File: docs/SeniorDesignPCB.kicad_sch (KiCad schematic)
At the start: 22 parts, among them J1 Conn_02x05_Odd_Even, SW1 RotaryEncoder_Switch, SW2 RotaryEncoder_Switch, SW3 SW_Push, U2 STM32F446RETx, U3 RC1602A, U4 MAX7375AXR805

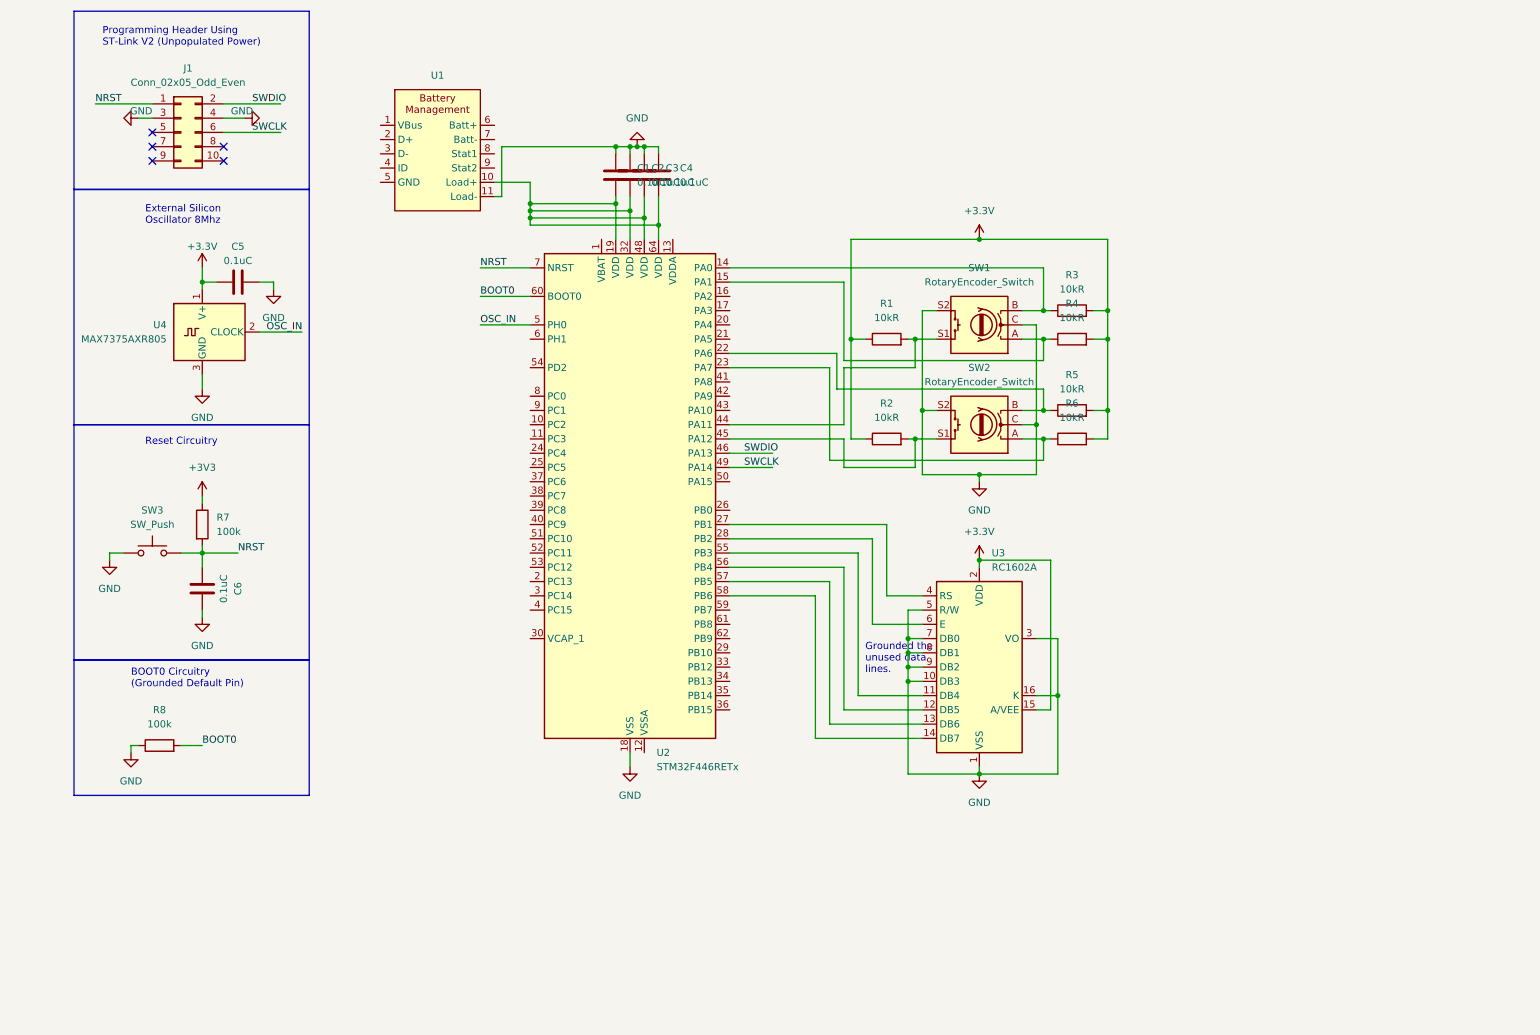
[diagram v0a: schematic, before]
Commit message: Add files via upload
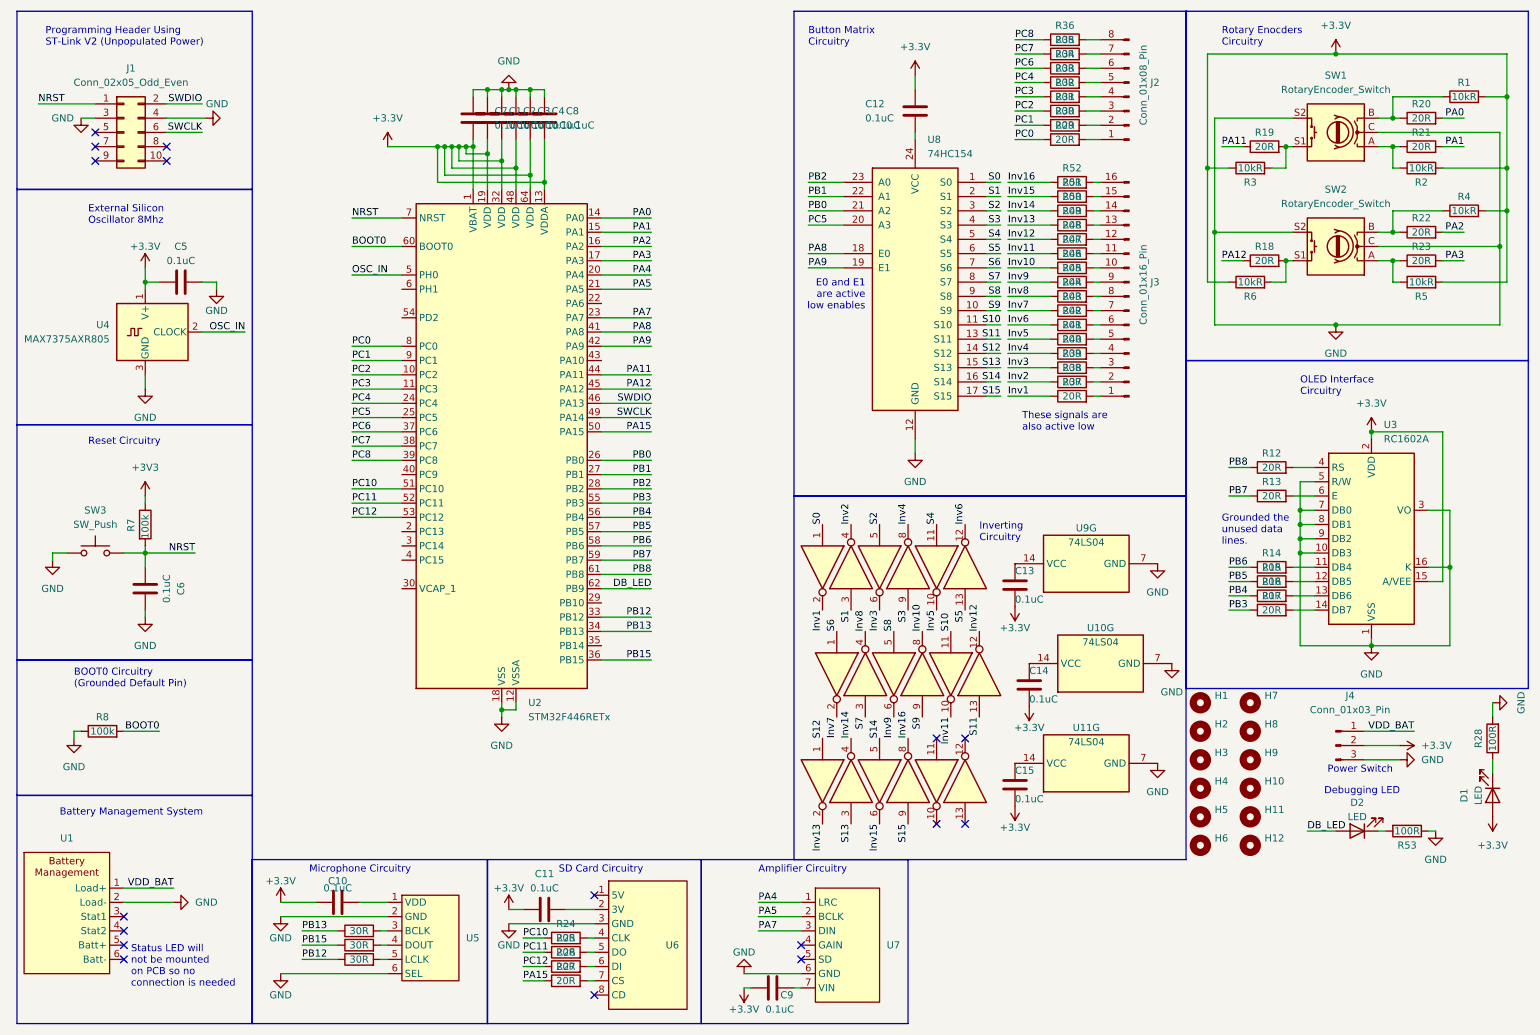
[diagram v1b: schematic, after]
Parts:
- added C10, C11, C12, C13, C14, C15, C7, C8, C9: 0.1uC, Capacitor_SMD:C_0805_2012Metric_Pad1.18x1.45mm_HandSolder, symbol Device:C
- added D1: LED, Diode_THT:D_5KP_P7.62mm_Vertical_AnodeUp, symbol Device:LED
- added D2: LED, Diode_SMD:D_0805_2012Metric, symbol Device:LED
- added H1, H2, H3, H4, H5, H6, H7, H8: MountingHole, MountingHole:MountingHole_2.2mm_M2, symbol Mechanical:MountingHole
- added H10, H11, H12, H9: MountingHole, MountingHole:MountingHole_2.5mm, symbol Mechanical:MountingHole
- added J2: Conn_01x08_Pin, Connector_PinHeader_2.54mm:PinHeader_1x08_P2.54mm_Vertical, symbol Connector:Conn_01x08_Pin
- added J3: Conn_01x16_Pin, Connector_PinHeader_2.54mm:PinHeader_1x16_P2.54mm_Vertical, symbol Connector:Conn_01x16_Pin
- added J4: Conn_01x03_Pin, Connector_PinHeader_2.54mm:PinHeader_1x03_P2.54mm_Vertical, symbol Connector:Conn_01x03_Pin
- added R10, R11, R9: 30R, Resistor_SMD:R_0805_2012Metric_Pad1.20x1.40mm_HandSolder, symbol Device:R
- added R12, R13, R14, R15, R16, R17, R18, R19, R20, R21, R22, R23, R24, R25, R26, R27, R29, R30, R31, R32, R33, R34, R35, R36, R37, R38, R39, R40, R41, R42, R43, R44, R45, R46, R47, R48, R49, R50, R51, R52: 20R, Resistor_SMD:R_0805_2012Metric_Pad1.20x1.40mm_HandSolder, symbol Device:R
- added R28, R53: 100R, Resistor_SMD:R_0805_2012Metric_Pad1.20x1.40mm_HandSolder, symbol Device:R
- added U10, U11, U9: 74LS04, Package_DIP:DIP-14_W7.62mm, symbol 74xx:74LS04
- added U5: ~, Connector_PinHeader_2.54mm:PinHeader_1x06_P2.54mm_Vertical, symbol SeniorDesignLibrary:MicrophoneBreakout
- added U6: ~, Connector_PinHeader_2.54mm:PinHeader_1x08_P2.54mm_Vertical, symbol SeniorDesignLibrary:SDBreakout
- added U7: ~, Connector_PinHeader_2.54mm:PinHeader_1x07_P2.54mm_Vertical, symbol SeniorDesignLibrary:Amplifier
- added U8: 74HC154, Package_DIP:DIP-24_W7.62mm, symbol 74xx:74LS154
- C1, C2, C3, C4, C5, C6: footprint Capacitor_SMD:C_1206_3216Metric_Pad1.33x1.80mm_HandSolder -> Capacitor_SMD:C_0805_2012Metric_Pad1.18x1.45mm_HandSolder
- J1: footprint Connector_PinHeader_1.00mm:PinHeader_2x05_P1.00mm_Vertical -> Connector_PinHeader_2.54mm:PinHeader_2x05_P2.54mm_Vertical
- SW3: footprint (none) -> Button_Switch_SMD:SW_Push_1P1T_NO_6x6mm_H9.5mm
- U1: footprint SeniorDesignFPLibrary:PCB_BatteryManagement -> Connector_PinHeader_2.54mm:PinHeader_1x06_P2.54mm_Vertical
- U3: footprint Display:RC1602A -> Connector_PinHeader_2.54mm:PinHeader_1x16_P2.54mm_Vertical
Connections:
- net +3.3V: now also C1.2, C2.2, C3.2, C4.2, R1.2, R2.2, R3.1, R6.1, U2.1 (VBAT), U2.13 (VDDA), U2.19 (VDD), U2.32 (VDD), U2.48 (VDD), U2.64 (VDD), C10.1, C11.1, C12.1, C13.2, C14.2, C15.2, C7.2, C8.2, C9.1, D1.2 (A), J4.2 (Pin_2); no longer R1.1, R2.1, R3.2, R6.2
- net GND: now also U1.2 (Load-), U2.12 (VSSA), C7.1, C8.1, J4.3 (Pin_3), R28.2, R53.1, U10.7 (GND), U11.7 (GND), U5.2 (GND), U5.6 (SEL), U6.3 (GND), U7.6 (GND), U8.12 (GND), U9.7 (GND); no longer U1.11 (Load-)
- net PC2: now reaches U2.10 (PC2)
- net PC2: now also R31.1
- net PC3: now reaches U2.11 (PC3)
- net PC3: now also R32.1
- net PA2: now reaches U2.16 (PA2)
- net PA2: now also R22.2
- net PA3: now reaches U2.17 (PA3)
- net PA3: now also R23.2
- net PA4: now reaches U2.20 (PA4)
- net PA4: now also U7.1 (LRC)
- net PA5: now reaches U2.21 (PA5)
- net PA5: now also U7.2 (BCLK)
- net PC4: now reaches U2.24 (PC4)
- net PC4: now also R33.1
- net PC5: now reaches U2.25 (PC5)
- net PC5: now also U8.20 (A3)
- net PB0: now reaches U2.26 (PB0)
- net PB0: now also U8.21 (A2)
- net at U3.4 (RS): now also R12.2; no longer U2.27 (PB1)
- net at U3.6 (E): now also R13.2; no longer U2.28 (PB2)
- net PB12: now reaches U2.33 (PB12)
- net PB12: now also R11.1
- net PB13: now reaches U2.34 (PB13)
- net PB13: now also R9.1
- net PB15: now reaches U2.36 (PB15)
- net PB15: now also R10.1
- net PC6: now reaches U2.37 (PC6)
- net PC6: now also R34.1
- net PC7: now reaches U2.38 (PC7)
- net PC7: now also R35.1
- net PC8: now reaches U2.39 (PC8)
- net PC8: now also R36.1
- net PA8: now reaches U2.41 (PA8)
- net PA8: now also U8.18 (E0)
- net PA9: now reaches U2.42 (PA9)
- net PA9: now also U8.19 (E1)
- net PA15: now reaches U2.50 (PA15)
- net PA15: now also R27.1
- net PC10: now reaches U2.51 (PC10)
- net PC10: now also R24.1
- net PC11: now reaches U2.52 (PC11)
- net PC11: now also R25.1
- net PC12: now reaches U2.53 (PC12)
- net PC12: now also R26.1
- net at U3.11 (DB4): now also R14.2; no longer U2.55 (PB3)
- net at U3.12 (DB5): now also R15.2; no longer U2.56 (PB4)
- net at U3.13 (DB6): now also R16.2; no longer U2.57 (PB5)
- net at U3.14 (DB7): now also R17.2; no longer U2.58 (PB6)
- net PB7: now reaches U2.59 (PB7)
- net PB7: now also R13.1
- net PB8: now reaches U2.61 (PB8)
- net PB8: now also R12.1
- net DB_LED: now reaches U2.62 (PB9)
- net DB_LED: now also D2.2 (A)
- net PC0: now reaches U2.8 (PC0)
- net PC0: now also R29.1
- net PC1: now reaches U2.9 (PC1)
- net PC1: now also R30.1
- net VDD_BAT: now reaches U1.1 (Load+)
- net VDD_BAT: now also J4.1 (Pin_1)
- new net: R19.2, R3.2, SW1.S1
- new net: J3.5 (Pin_5), R41.2
- new net: R22.1, R4.1, SW2.B
- new net: R24.2, U6.4 (CLK)
- new net: R27.2, U6.7 (CS)
- new net: J2.4 (Pin_4), R32.2
- new net: J3.1 (Pin_1), R37.2
- new net: J3.10 (Pin_10), R46.2
- new net: J3.11 (Pin_11), R47.2
- new net: J3.12 (Pin_12), R48.2
- new net: J3.13 (Pin_13), R49.2
- new net: J3.14 (Pin_14), R50.2
- new net: J3.15 (Pin_15), R51.2
- new net: J3.16 (Pin_16), R52.2
- new net: J3.2 (Pin_2), R38.2
- new net: J3.3 (Pin_3), R39.2
- new net: J3.4 (Pin_4), R40.2
- new net: J3.6 (Pin_6), R42.2
- new net: J3.7 (Pin_7), R43.2
- new net: J3.8 (Pin_8), R44.2
- new net: J3.9 (Pin_9), R45.2
- new net: C10.2, U5.1 (VDD)
- new net: J2.1 (Pin_1), R29.2
- new net: J2.2 (Pin_2), R30.2
- new net: J2.3 (Pin_3), R31.2
- new net: J2.5 (Pin_5), R33.2
- new net: J2.6 (Pin_6), R34.2
- new net: J2.7 (Pin_7), R35.2
- new net: J2.8 (Pin_8), R36.2
- new net: D2.1 (K), R53.2
- new net: R11.2, U5.5 (LCLK)
- new net: C14.1, U10.14 (VCC)
- new net: C12.2, U8.24 (VCC)
- new net: R23.1, R5.1, SW2.A
- new net: R18.2, R6.2, SW2.S1
- new net: R2.1, R21.1, SW1.A
- new net: R1.1, R20.1, SW1.B
- new net: D1.1 (K), R28.1
- new net: C9.2, U7.7 (VIN)
- new net: R25.2, U6.5 (DO)
- new net: C11.2, U6.2 (3V)
- new net: R26.2, U6.6 (DI)
- new net: R9.2, U5.3 (BCLK)
- new net: R10.2, U5.4 (DOUT)
- new net: C13.1, U9.14 (VCC)
- new net: C15.1, U11.14 (VCC)
- new net Inv1: R37.1, U9.2
- new net Inv10: R46.1, U10.8
- new net Inv11: R47.1, U10.10
- new net Inv12: R48.1, U10.12
- new net Inv13: R49.1, U11.2
- new net Inv14: R50.1, U11.4
- new net Inv15: R51.1, U11.6
- new net Inv16: R52.1, U11.8
- new net Inv2: R38.1, U9.4
- new net Inv3: R39.1, U9.6
- new net Inv4: R40.1, U9.8
- new net Inv5: R41.1, U9.10
- new net Inv6: R42.1, U9.12
- new net Inv7: R43.1, U10.2
- new net Inv8: R44.1, U10.4
- new net Inv9: R45.1, U10.6
- new net PA0: R20.2, U2.14 (PA0)
- new net PA1: R21.2, U2.15 (PA1)
- new net PA11: R19.1, U2.44 (PA11)
- new net PA12: R18.1, U2.45 (PA12)
- new net PA7: U2.23 (PA7), U7.3 (DIN)
- new net PB1: U2.27 (PB1), U8.22 (A1)
- new net PB2: U2.28 (PB2), U8.23 (A0)
- new net PB3: R17.1, U2.55 (PB3)
- new net PB4: R16.1, U2.56 (PB4)
- new net PB5: R15.1, U2.57 (PB5)
- new net PB6: R14.1, U2.58 (PB6)
- new net S0: U8.1 (S0), U9.1
- new net S1: U8.2 (S1), U9.3
- new net S10: U10.11, U8.11 (S10)
- new net S11: U10.13, U8.13 (S11)
- new net S12: U11.1, U8.14 (S12)
- new net S13: U11.3, U8.15 (S13)
- new net S14: U11.5, U8.16 (S14)
- new net S15: U11.9, U8.17 (S15)
- new net S2: U8.3 (S2), U9.5
- new net S3: U8.4 (S3), U9.9
- new net S4: U8.5 (S4), U9.11
- new net S5: U8.6 (S5), U9.13
- new net S6: U10.1, U8.7 (S6)
- new net S7: U10.3, U8.8 (S7)
- new net S8: U10.5, U8.9 (S8)
- new net S9: U10.9, U8.10 (S9)
- now unconnected: U2.22 (PA6)
- no-connect marks 5 -> 17
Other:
- note added: "Amplifier Circuitry"
- note added: "Battery Management System"
- note added: "Button Matrix Circuitry"
- note added: "Debugging LED"
- note added: "E0 and E1 are active low enables"
- note added: "Inverting Circuitry"
- note added: "Microphone Circuitry"
- note added: "OLED Interface Circuitry"
- note added: "Power Switch"
- note added: "Rotary Enocders Circuitry"
- note added: "SD Card Circuitry"
- note added: "Status LED will not be mounted on PCB so no connection is needed"
- note added: "These signals are also active low"
- moved on the sheet: C1, C2, C3, C4, C5, C6, J1, R1, R2, R3, R4, R5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
